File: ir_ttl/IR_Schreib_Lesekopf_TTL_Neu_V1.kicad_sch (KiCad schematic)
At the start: 18 parts, among them IC1 74LVC1G17DBVR, IC2 74LVC1G17DBVR, T1 SFH309FA-4, T2 BC807-40, T3 BC817-40, X1 +UB, X2 TXD, X3 RXD, X4 GND

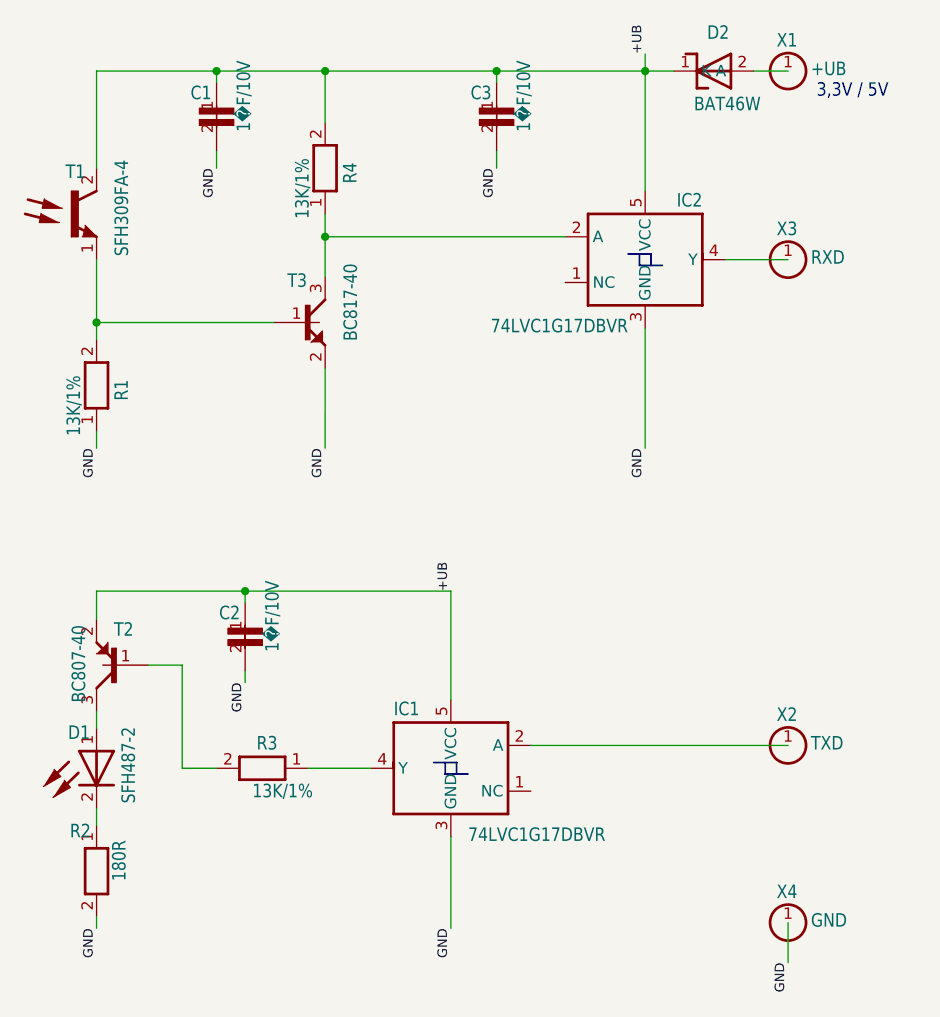
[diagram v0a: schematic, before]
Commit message: updated some footprints and cutouts WIP
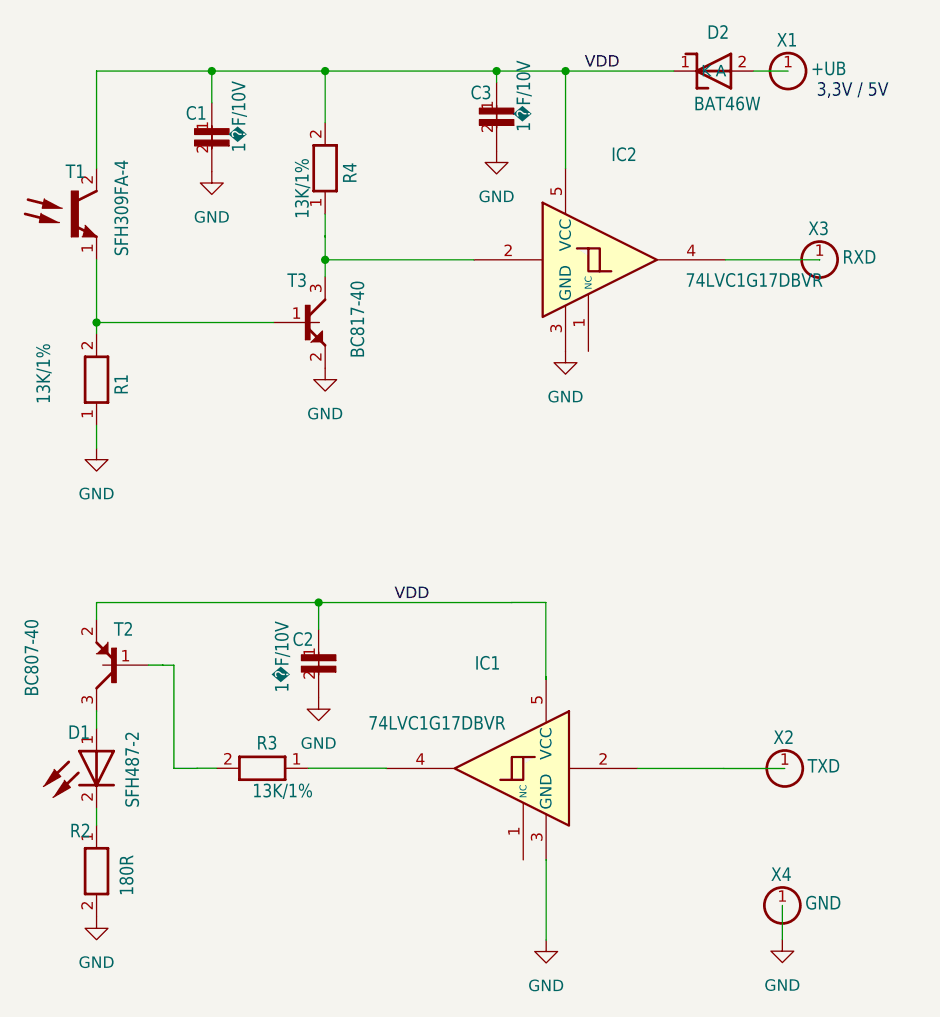
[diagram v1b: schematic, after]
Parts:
- IC1, IC2: footprint IR_Schreib_Lesekopf_TTL_Neu_V1:SOT23_5 -> Package_TO_SOT_SMD:SOT-23-5; symbol IR_Schreib_Lesekopf_TTL_Neu_V1-eagle-import:74LVC1G17DBVR -> 74xGxx:74LVC1G17
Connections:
- net +UB renamed VDD
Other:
- moved on the sheet: C1, C2, R1, X2, X3, X4
